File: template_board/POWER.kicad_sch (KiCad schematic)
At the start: 31 parts, among them IC3 LMR16030SDDAR, J2 Conn_01x02, J6 Conn_01x02, U4 AZ1117-3.3

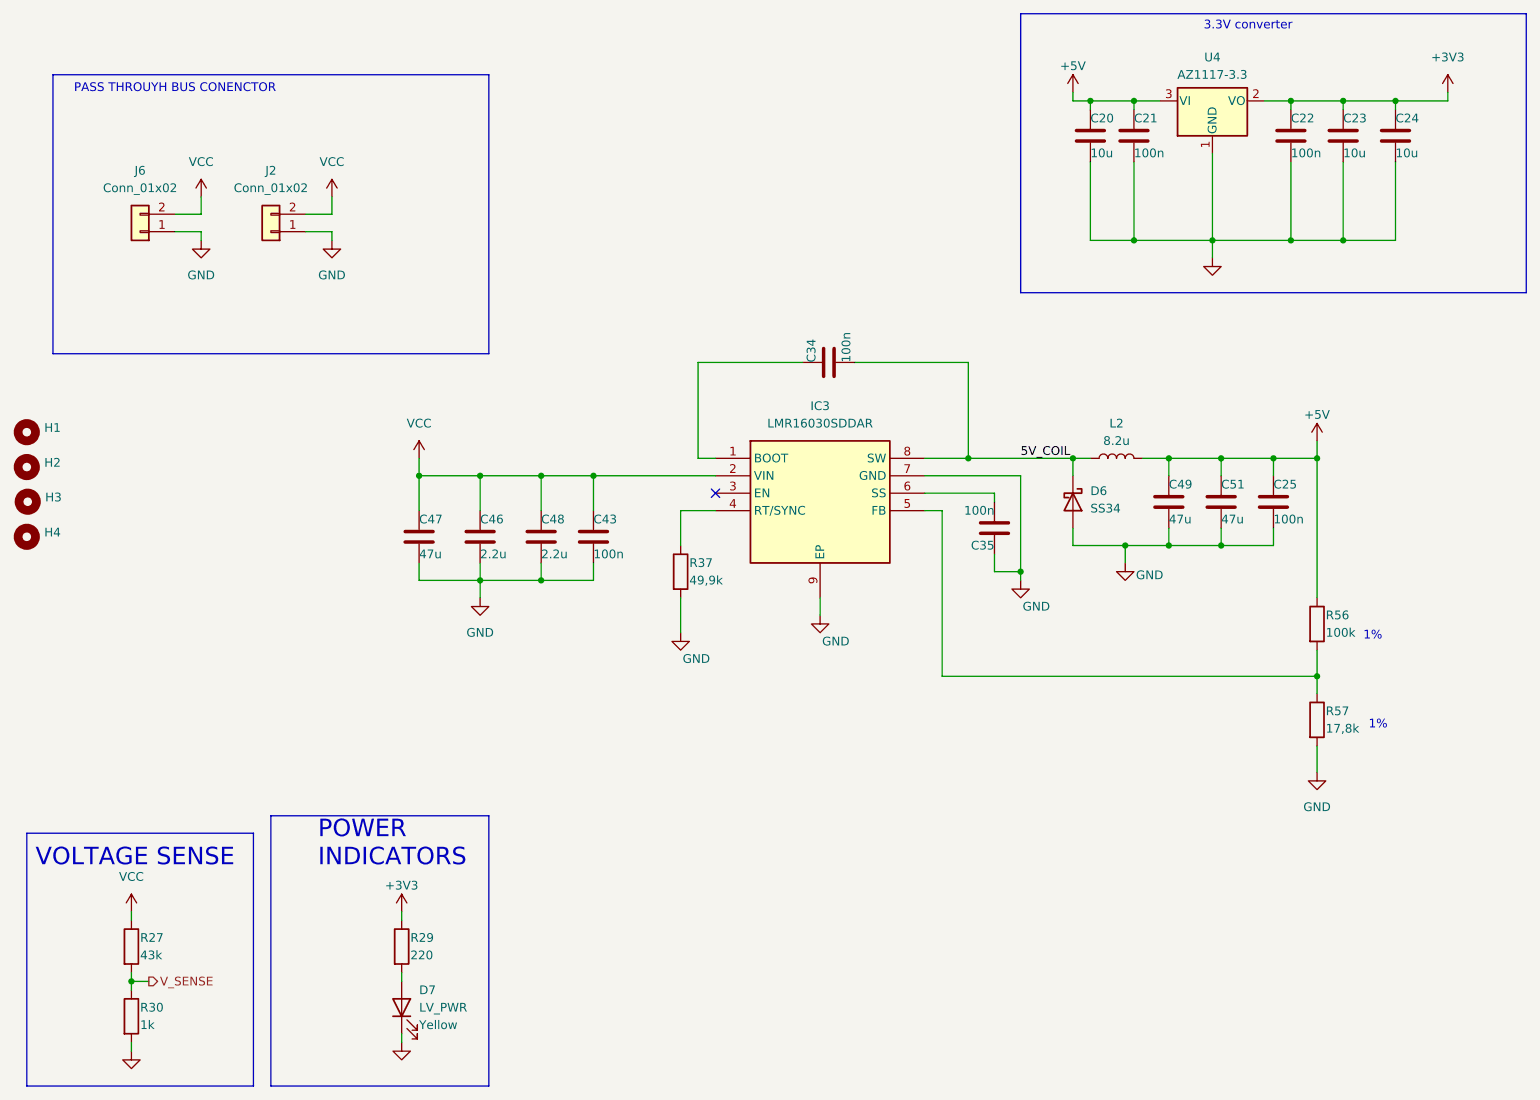
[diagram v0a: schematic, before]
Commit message: u5 wip
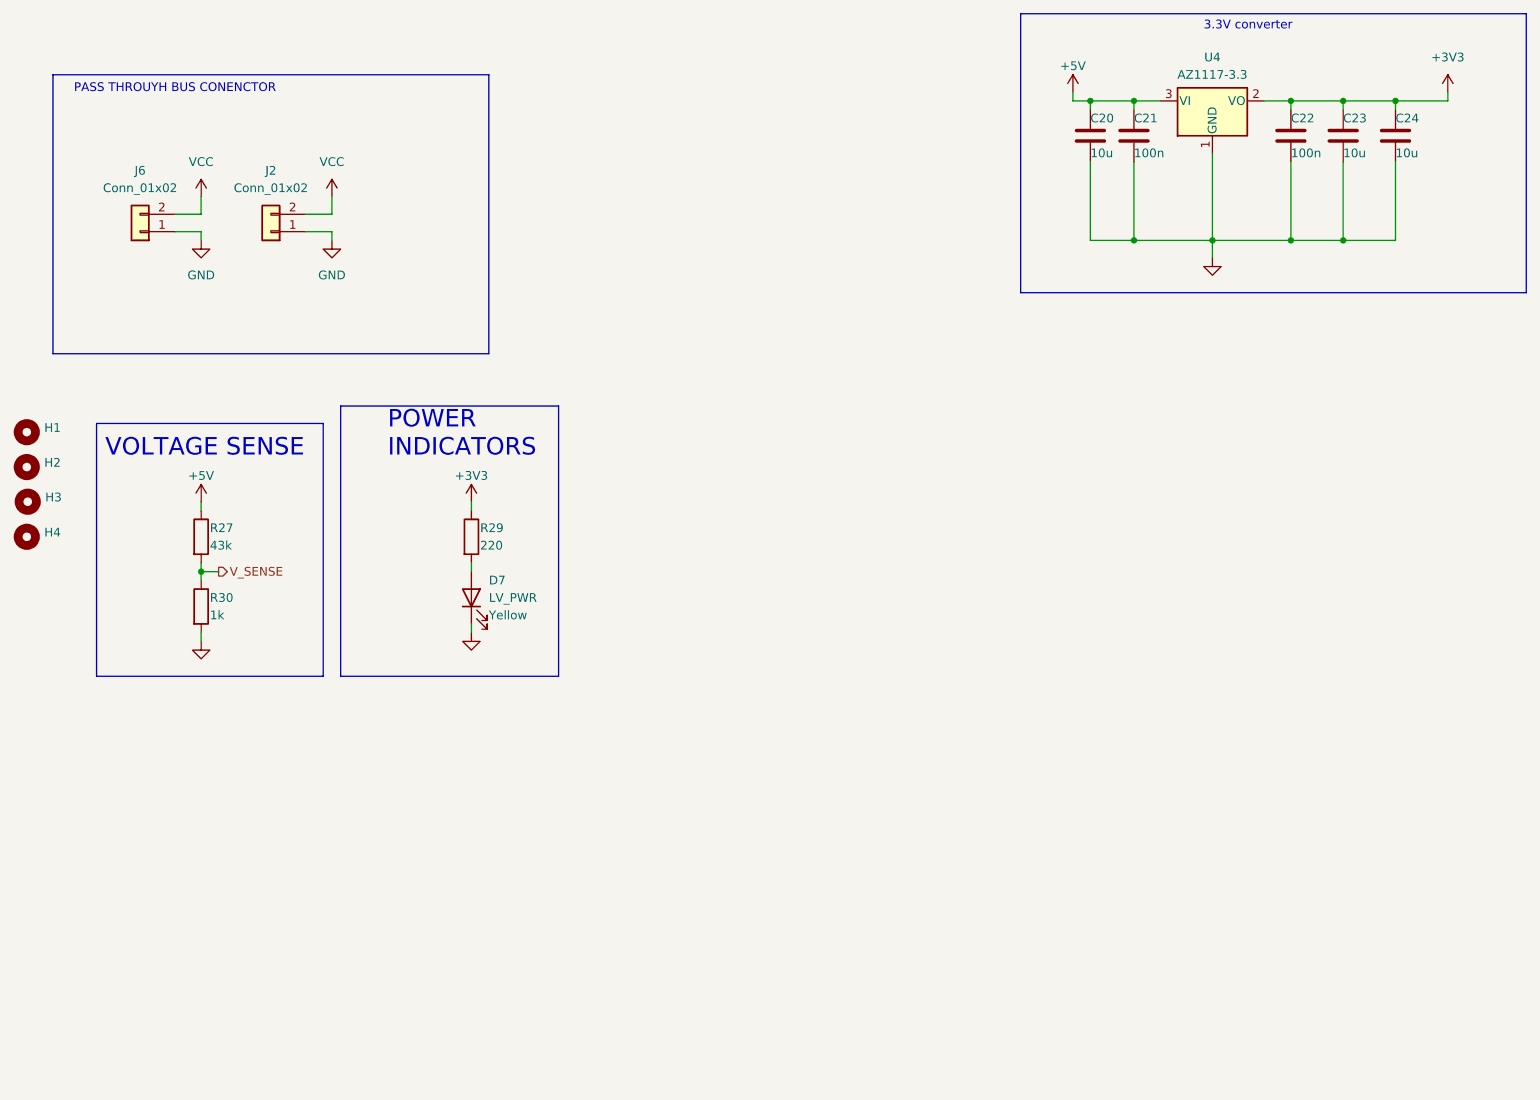
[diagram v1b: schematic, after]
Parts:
- removed C25, C34, C35, C43: 100n, Capacitor_SMD:C_0402_1005Metric, symbol Device:C
- removed C46, C48: 2.2u, Capacitor_SMD:C_1206_3216Metric, symbol Device:C
- removed C47: 47u, Capacitor_SMD:C_Elec_10x10.2, symbol Device:C
- removed C49, C51: 47u, Capacitor_SMD:C_1206_3216Metric, symbol Device:C
- removed D6: SS34, Diode_SMD:D_SMA, symbol Diode:SS34
- removed IC3: LMR16030SDDAR, parts:SOIC127P600X170-9N, symbol LMR16030SDDAR:LMR16030SDDAR
- removed L2: 8.2u, Inductor_SMD:L_Cenker_CKCS6045, symbol Device:L
- removed R37: 49,9k, Resistor_SMD:R_0402_1005Metric, symbol Device:R
- removed R56: 100k, Resistor_SMD:R_0402_1005Metric, symbol Device:R
- removed R57: 17,8k, Resistor_SMD:R_0402_1005Metric, symbol Device:R
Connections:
- net +5V: now also R27.1
- net VCC: no longer R27.1
- no-connect marks 1 -> 0
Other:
- note removed: "1%"
- moved on the sheet: D7, R27, R29, R30
